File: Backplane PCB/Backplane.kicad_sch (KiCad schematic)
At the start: 213 parts, among them J1 10018783-10202TLF, J2 10018783-10202TLF, J3 10018783-10202TLF, J4 10018783-10202TLF, J5 10018783-10202TLF, J6 5019514000, U1 LTC3894EFE-PBF, U10 ADP7104ACPZ-R7, U11 ISP817CXSM, U12 ISP817CXSM, U13 ISP817CXSM, U14 ISP817CXSM, U15 ISP817CXSM, U16 ISP817CXSM, U17 OP191GSZ-REEL7, U18 OP191GSZ-REEL7, U19 OP191GSZ-REEL7, U2 FDS4435A, U20 OP191GSZ-REEL7, U21 OP191GSZ-REEL7, U3 ISP817CXSM, U4 ISP817CXSM, U5 ISP817CXSM, U6 ISP817CXSM, U7 ISP817CXSM, U8 ISP817CXSM, U9 ADP7104ACPZ-R7

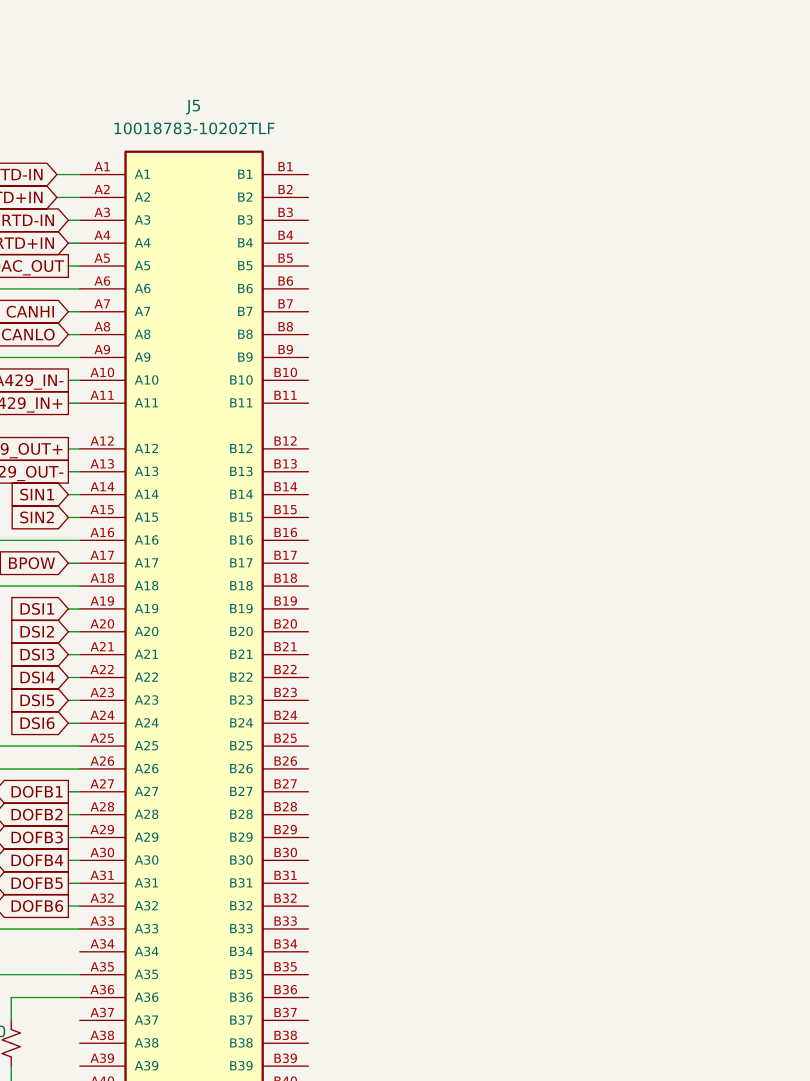
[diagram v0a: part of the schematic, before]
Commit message: Added logo
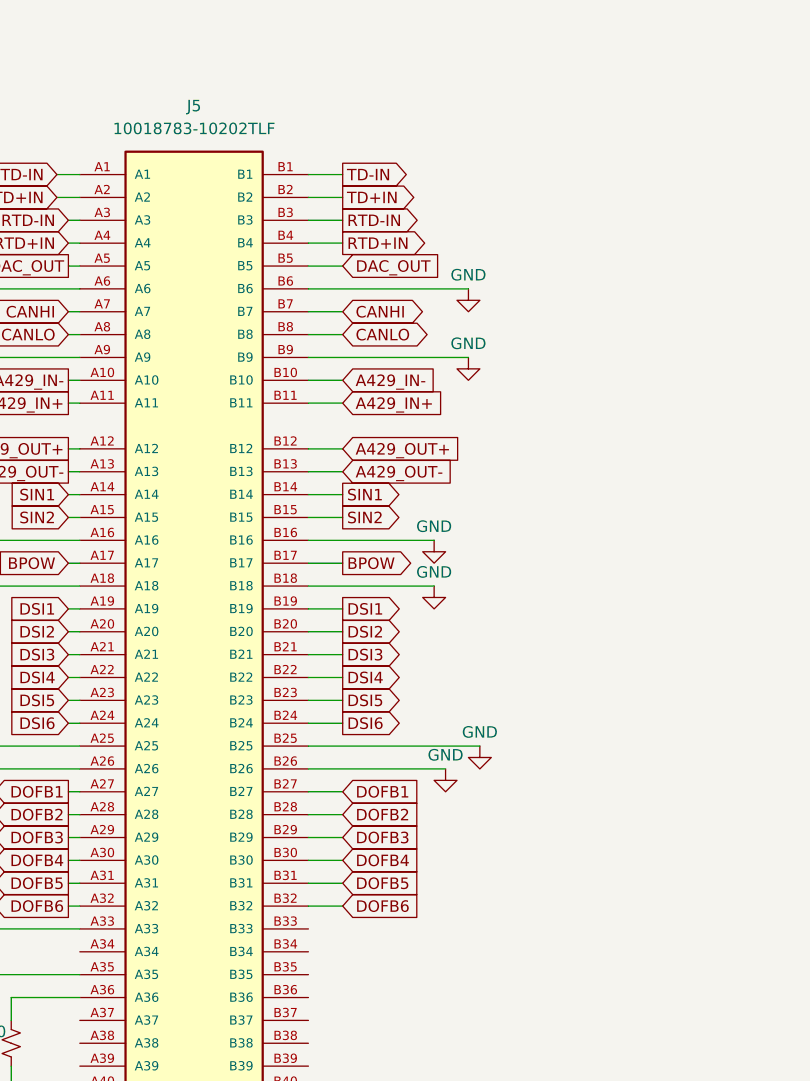
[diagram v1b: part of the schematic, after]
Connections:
- net A429_IN+: now also J5.B11
- net A429_IN-: now also J5.B10
- net A429_OUT+: now also J5.B12
- net A429_OUT-: now also J5.B13
- net BPOW: now also J5.B17
- net CANHI: now also J5.B7
- net CANLO: now also J5.B8
- net DAC_OUT: now also J5.B5
- net DOFB1: now also J5.B27
- net DOFB2: now also J5.B28
- net DOFB3: now also J5.B29
- net DOFB4: now also J5.B30
- net DOFB5: now also J5.B31
- net DOFB6: now also J5.B32
- net DSI1: now also J5.B19
- net DSI2: now also J5.B20
- net DSI3: now also J5.B21
- net DSI4: now also J5.B22
- net DSI5: now also J5.B23
- net DSI6: now also J5.B24
- net GND: now also J5.B16, J5.B18, J5.B25, J5.B26, J5.B6, J5.B9
- net RTD+IN: now also J5.B4
- net RTD-IN: now also J5.B3
- net SIN1: now also J5.B14
- net SIN2: now also J5.B15
- net TD+IN: now also J5.B2
- net TD-IN: now also J5.B1
